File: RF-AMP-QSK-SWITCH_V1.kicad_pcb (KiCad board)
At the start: 2 copper layers, 100 x 160 mm, 200 parts, among them J1 TRX, J2 AMP_IN, J3 ANT, J4 AMP_OUT, J5 Screw_Terminal_01x08, Q1 BCP56, Q10 PBHV2160Z, Q11 BC857, Q12 MMBTA92, Q13 MMBTA92, Q14 BC817, Q15 MMBTA92, Q16 MMBTA92, Q17 MMBTA92, Q18 MMBTA92, Q19 MMBTA42, Q2 STN9260, Q20 BC857, Q21 BC817, Q22 BC857, Q23 BC817, Q24 BC857, Q25 BC817, Q26 BC817, Q3 STN9260, Q4 BC817, Q5 STN9260, Q6 STN9260, Q7 STN9260, Q8 STN9260, Q9 STN9260, U1 LM2576S-ADJ, U2 L78L12_SOT89, U3 LT1963AEQ

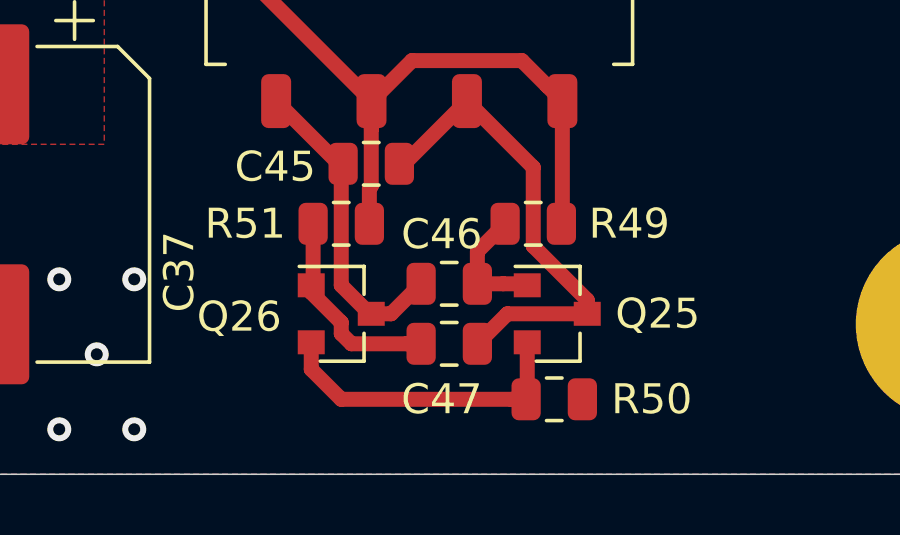
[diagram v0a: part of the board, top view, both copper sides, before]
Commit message: Revision1
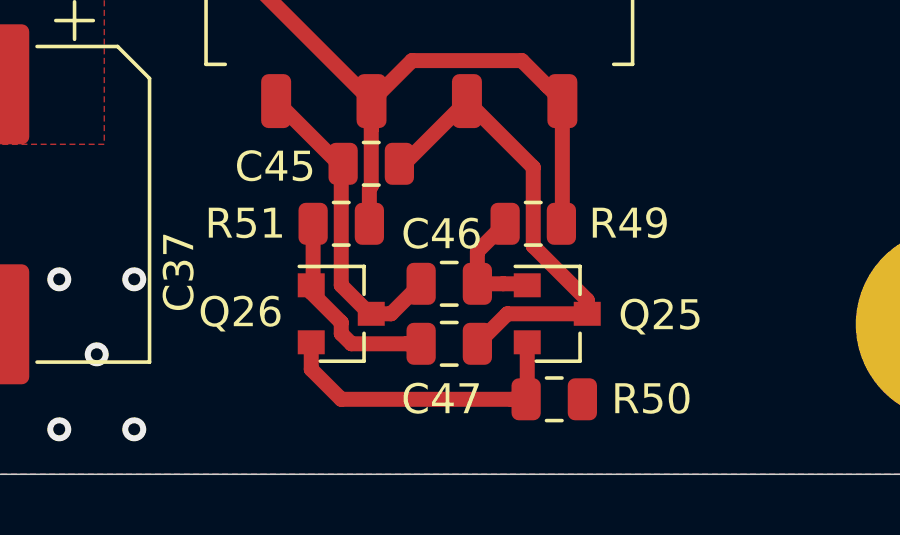
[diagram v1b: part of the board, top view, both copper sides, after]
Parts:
- C33, C59: value 470n -> 100n
- C36, C41, C42, C43, C44, C48, C49, C50, C51, C52, C53, C54, C55, C56: value 100n -> 1n
- C45: value 82n -> 470p
- L11: value 10u -> 68u
- Q25, Q26: value BC817 -> BSS138
- R14: value 1R5 -> 1
- R39: value 1M -> 100k
- R44: value 470k -> 100k
- R50: value 33 -> 0
- R52: value 3R3 -> 1k8
- R53: value 3R3 -> 3k3
